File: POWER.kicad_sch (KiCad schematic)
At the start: 26 parts, among them J14 USB_C_Receptacle_USB2.0_16P, U10 REF3033, U11 RY8411, U12 XC6210B332MR, U9 USBLC6-2SC6

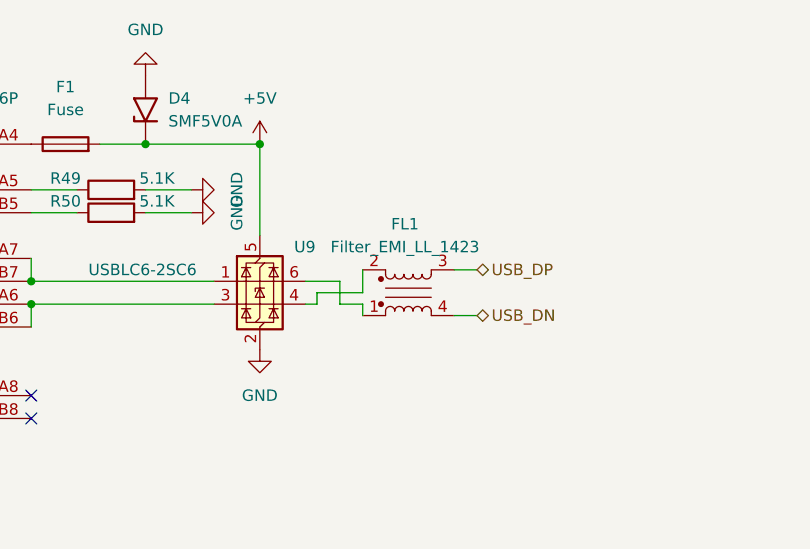
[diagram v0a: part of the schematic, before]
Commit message: Update KiCad project files
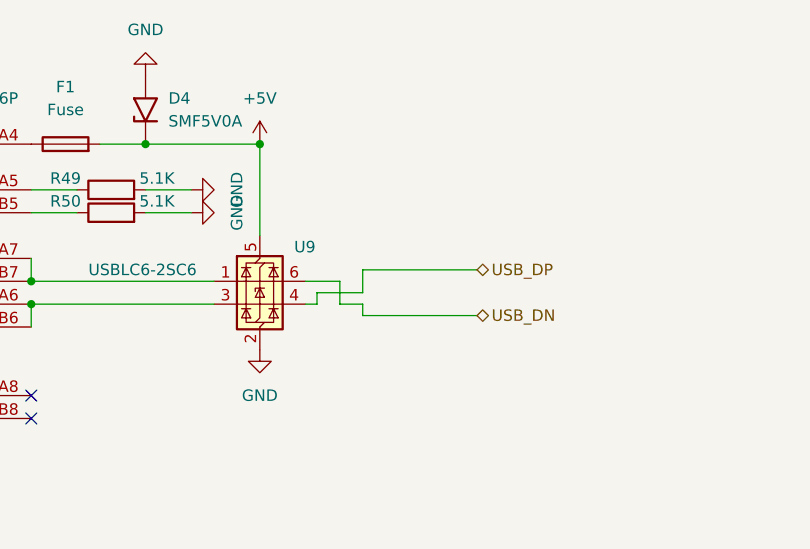
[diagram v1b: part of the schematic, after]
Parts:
- removed FL1: Filter_EMI_LL_1423, Inductor_SMD:L_CommonModeChoke_Coilank_ACM2012, symbol Device:Filter_EMI_LL_1423
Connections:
- net USB_DN: now also U9.6 (I/O1)
- net USB_DP: now also U9.4 (I/O2)
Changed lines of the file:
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@@
-	(wire
-		(pts
-			(xy 109.22 69.85) (xy 106.68 69.85)
-		)
-		(stroke
-			(width 0)
-			(type default)
-		)
-	)
 	(wire
 		(pts
@@
 	(wire
 		(pts
+			(xy 96.52 69.85) (xy 109.22 69.85)
+		)
+		(stroke
+			(width 0)
+			(type default)
+		)
+	)
+	(wire
+		(pts
 			(xy 93.98 68.58) (xy 96.52 68.58)
 		)
@@
 	(wire
 		(pts
-			(xy 109.22 64.77) (xy 106.68 64.77)
-		)
-		(stroke
-			(width 0)
-			(type default)
-		)
-	)
-	(wire
-		(pts
 			(xy 171.45 50.8) (xy 171.45 66.04)
 		)
@@
 		(pts
 			(xy 176.53 60.96) (xy 172.72 60.96)
+		)
+		(stroke
+			(width 0)
+			(type default)
+		)
+	)
+	(wire
+		(pts
+			(xy 96.52 64.77) (xy 109.22 64.77)
 		)
 		(stroke
@@
 					(unit 1)
 				)
-			)
-		)
-	)
-	(symbol
-		(lib_id "Device:Filter_EMI_LL_1423")
-		(at 101.6 67.31 0)
-		(unit 1)
-		(body_style 1)
-		(exclude_from_sim no)
-		(in_bom yes)
-		(on_board yes)
-		(in_pos_files yes)
-		(dnp no)
-		(fields_autoplaced yes)
-		(property "Reference" "FL1"
-			(at 101.219 59.69 0)
-			(show_name no)
-			(do_not_autoplace no)
-			(effects
-				(font
-					(size 1.27 1.27)
-				)
-			)
-		)
-		(property "Value" "Filter_EMI_LL_1423"
-			(at 101.219 62.23 0)
-			(show_name no)
-			(do_not_autoplace no)
-			(effects
-				(font
-					(size 1.27 1.27)
-				)
-			)
-		)
-		(property "Footprint" "Inductor_SMD:L_CommonModeChoke_Coilank_ACM2012"
-			(at 101.6 73.66 0)
-			(hide yes)
-			(show_name no)
-			(do_not_autoplace no)
-			(effects
-				(font
-					(size 1.27 1.27)
-				)
-			)
-		)
-		(property "Datasheet" ""
-			(at 101.6 66.294 90)
-			(hide yes)
-			(show_name no)
-			(do_not_autoplace no)
-			(effects
-				(font
-					(size 1.27 1.27)
-				)
-			)
-		)
-		(property "Description" "EMI 2-inductor filter, pin-connections 1-4 and 2-3"
-			(at 101.6 67.31 0)
-			(hide yes)
-			(show_name no)
-			(do_not_autoplace no)
-			(effects
-				(font
-					(size 1.27 1.27)
-				)
-			)
-		)
-		(property "KLC_S3.3" ""
-			(at 101.6 67.31 0)
-			(hide yes)
-			(show_name no)
-			(do_not_autoplace no)
-			(effects
-				(font
-					(size 1.27 1.27)
-				)
-			)
-		)
-		(property "KLC_S4.1" ""
-			(at 101.6 67.31 0)
-			(hide yes)
-			(show_name no)
-			(do_not_autoplace no)
-			(effects
-				(font
-					(size 1.27 1.27)
-				)
-			)
-		)
-		(pin "4"
-		)
-		(pin "3"
-		)
-		(pin "2"
-		)
-		(pin "1"
-		)
-		(instances
-			(project "HPM5E31"
-				(path "/c97d420a-5bfd-40ab-9a74-5349ba6434d5/a6e05f59-c850-40f8-96e7-7ebc30b62383"
-					(reference "FL1")
-					(unit 1)
-				)
